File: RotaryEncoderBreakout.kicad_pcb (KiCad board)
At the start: 2 copper layers, 36 x 44.1 mm, 18 parts, among them J1 Conn_01x04_Male, J2 Conn_01x04_Male, J3 Conn_01x03_Male, SW1 RotaryEncoder_Switch_RGB, U1 WS2811

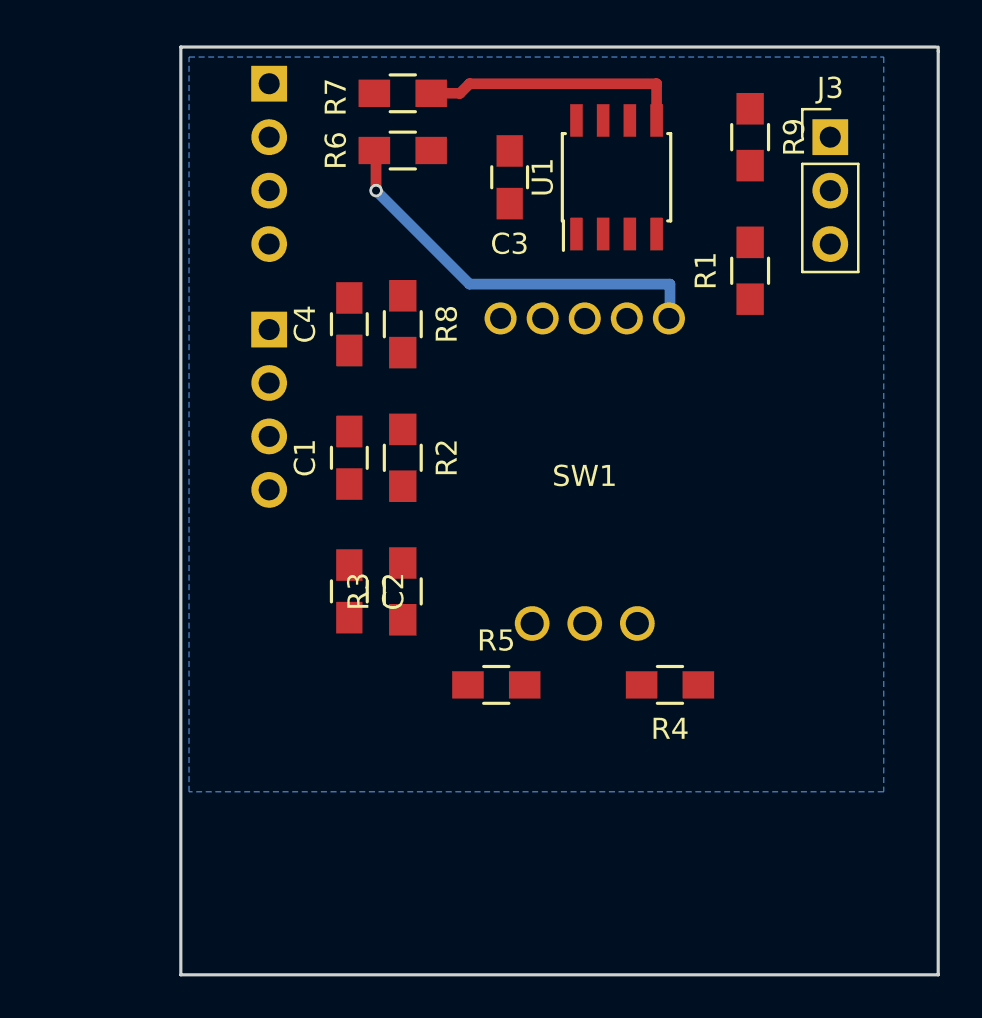
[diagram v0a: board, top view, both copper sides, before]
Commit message: Layout complete
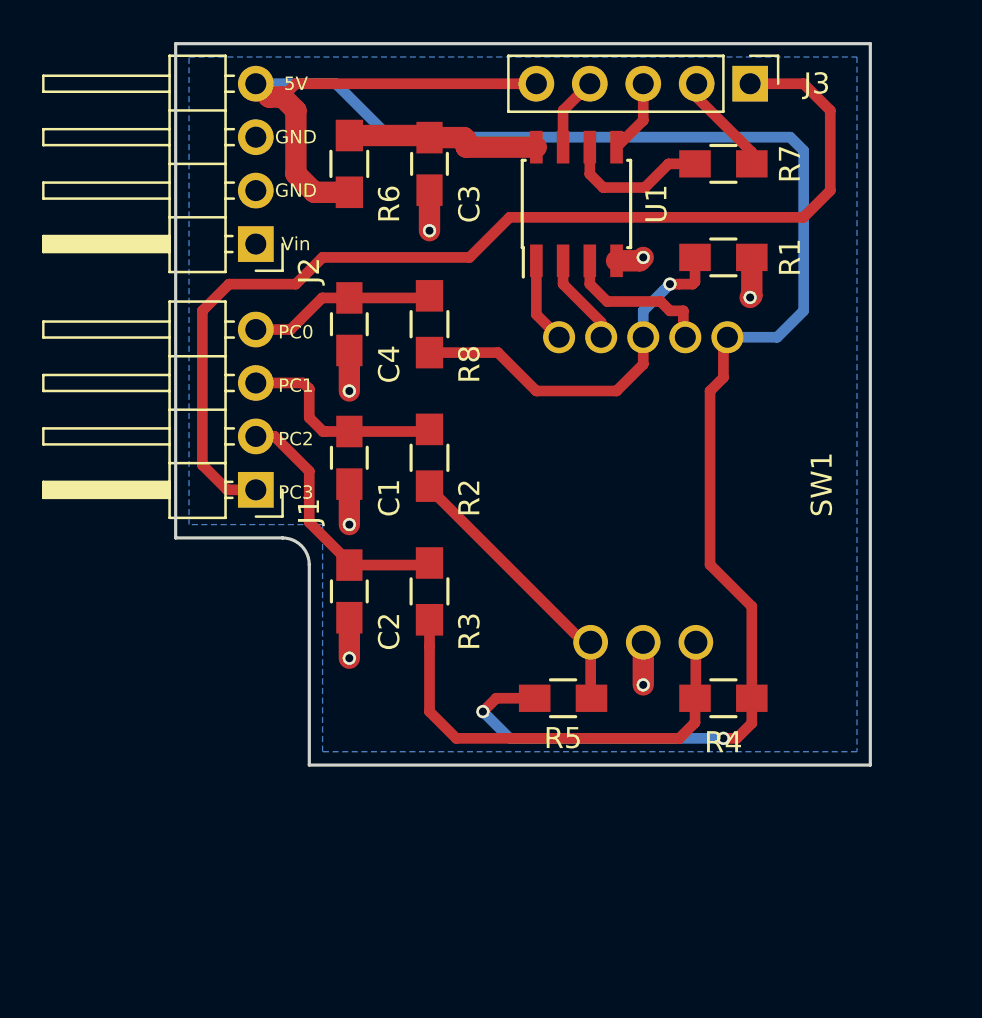
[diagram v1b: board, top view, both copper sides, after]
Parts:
- removed R9: 0R, Resistors_SMD:R_0805_HandSoldering
- J1, J2: moved to F.Cu
- J3: value Conn_01x03_Male -> Conn_01x05_Male; footprint Pin_Headers:Pin_Header_Straight_1x03_Pitch2.54mm -> Pin_Headers:Pin_Header_Straight_1x05_Pitch2.54mm
- moved R7 15.6 mm to (135.9, 59.1)
- moved J1 7.65 mm to (113.7, 74.5)
- moved J2 7.65 mm to (113.7, 62.9)
- moved J3 4.58 mm to (137.2, 55.2), turned to 270 degrees
- moved C3 3.86 mm to (121.9, 59.1)
- moved R5 3.24 mm to (128.3, 84.5)
- moved SW1 2.92 mm to (132.1, 74.3)
- moved R6 2.62 mm to (118.1, 59.1), turned to 90 degrees
- moved R4 2.62 mm to (135.9, 84.5)
- moved U1 2.29 mm to (128.9, 61.0)
- moved R1 1.42 mm to (135.9, 63.5), turned to 0 degrees
- moved R2 1.27 mm to (121.9, 73.0), turned to 90 degrees
- moved R3 1.27 mm to (121.9, 79.4)
- moved R8 1.27 mm to (121.9, 66.7), turned to 90 degrees
- turned C1 to 270 degrees
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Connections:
- J1 pad 1: Net-(C4-Pad1) -> Net-(J1-Pad1)
- J1 pad 2: Net-(C1-Pad1) -> Net-(C2-Pad1)
- J1 pad 3: Net-(C2-Pad1) -> Net-(C1-Pad1)
- J1 pad 4: Net-(J1-Pad4) -> Net-(C4-Pad1)
- J2 pad 1: +5V -> Net-(J2-Pad1)
- J2 pad 4: Net-(J2-Pad4) -> +5V
- J3 pad 1: Net-(J3-Pad1) -> Net-(J1-Pad1)
- J3 pad 3: Net-(J1-Pad4) -> Net-(J3-Pad3)
- U1 pad 5: Net-(J3-Pad1) -> Net-(J3-Pad3)
- U1 pad 7: Net-(R9-Pad2) -> Net-(J3-Pad4)
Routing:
- net +5V: track 19.4 -> 95.6 mm, vias 1 -> 2
- net Net-(J1-Pad1): track 0.00 -> 50.7 mm
- net Net-(R3-Pad1): track 0.00 -> 21.7 mm
- net Net-(R1-Pad1): track 0.00 -> 18.2 mm, vias 0 -> 1
- net Net-(R2-Pad1): track 0.00 -> 13.5 mm
- net GND: track 0.00 -> 13.0 mm, vias 0 -> 7
- net Net-(C2-Pad1): track 0.00 -> 12.3 mm
- net Net-(J3-Pad1): track 10.6 -> 0.00 mm
- net Net-(C1-Pad1): track 0.00 -> 10.1 mm
- net Net-(C3-Pad2): track 0.00 -> 9.33 mm
- net Net-(C4-Pad1): track 0.00 -> 8.92 mm
- net Net-(SW1-Pad4): track 0.00 -> 7.38 mm
- net Net-(R7-Pad1): track 0.00 -> 7.01 mm
- net Net-(SW1-Pad2): track 0.00 -> 4.38 mm
- net Net-(SW1-Pad1): track 0.00 -> 4.08 mm
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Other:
- board size 36 x 44.1 mm -> 33 x 34.3 mm
- board text added: "5V"
- board text added: "GND"
- board text added: "PC0"
- board text added: "PC1"
- board text added: "PC2"
- board text added: "PC3"
- board text added: "Vin"
